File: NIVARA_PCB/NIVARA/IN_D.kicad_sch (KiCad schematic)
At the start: 0 parts

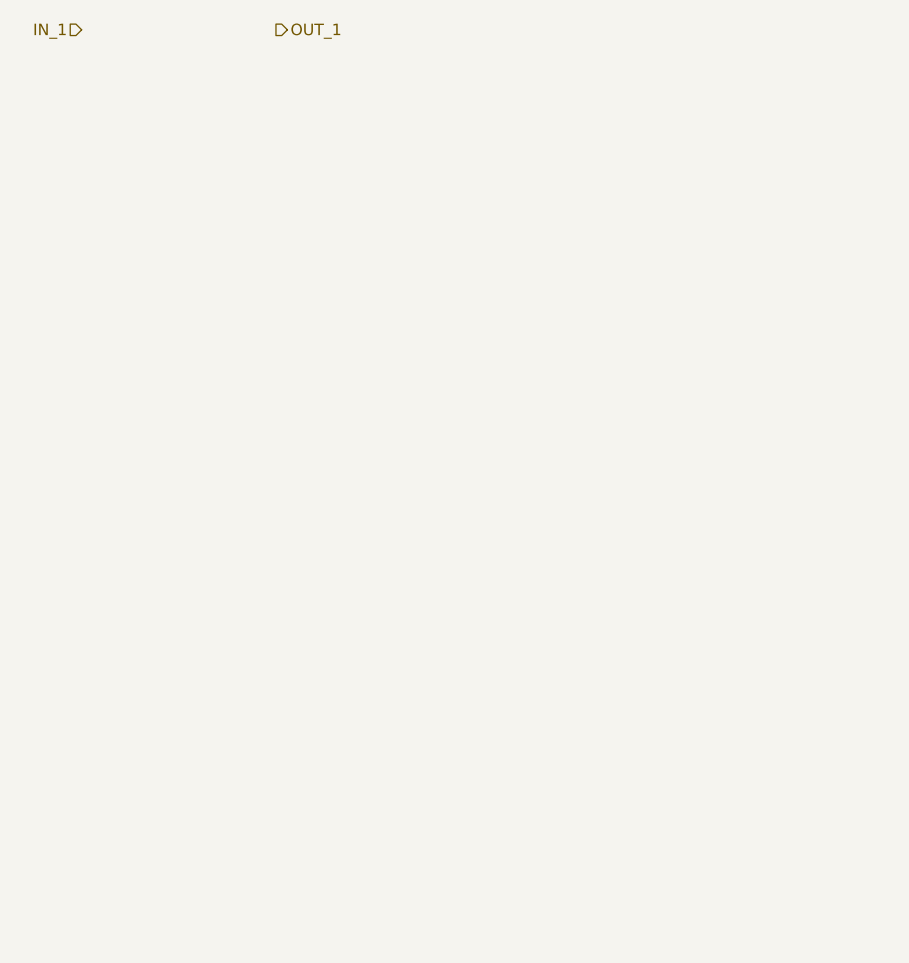
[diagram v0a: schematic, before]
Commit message: avance
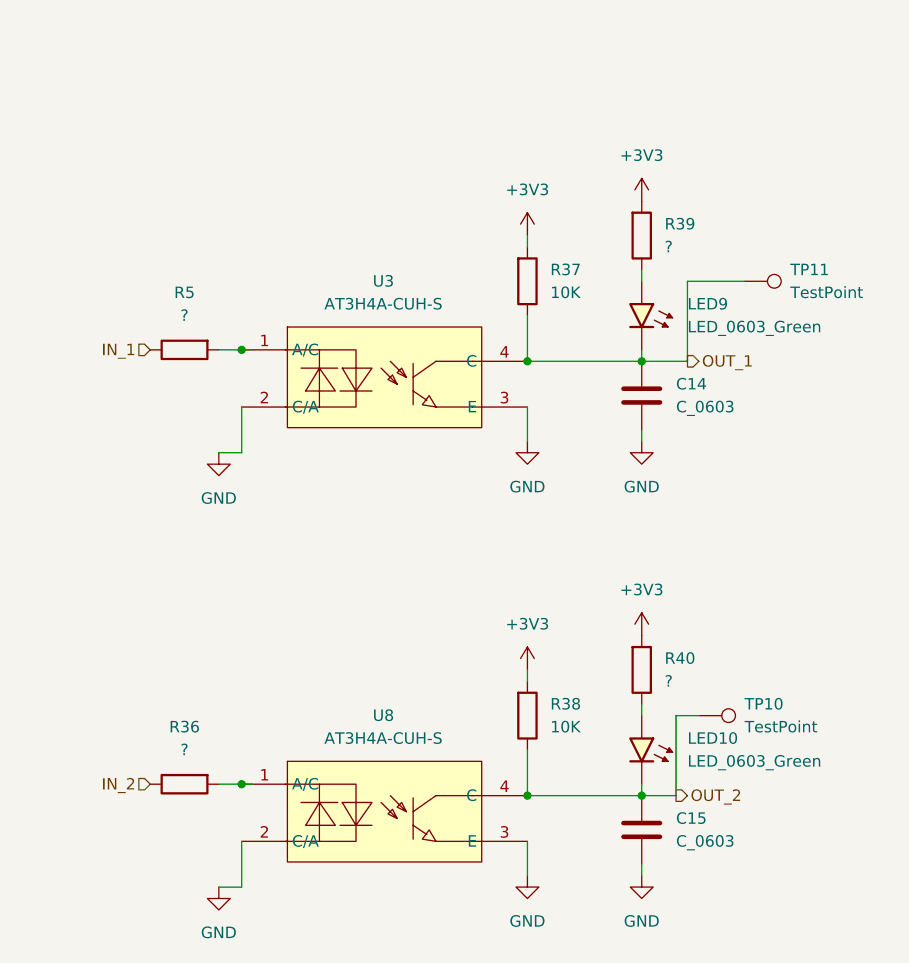
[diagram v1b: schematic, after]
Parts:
- added C14, C15: C_0603, PCM_Capacitor_SMD_AKL:C_0603_1608Metric, symbol PCM_Capacitor_AKL:C_0603
- added LED10, LED9: LED_0603_Green, PCM_LED_SMD_AKL:LED_0603_1608Metric, symbol PCM_LED_AKL:LED_0603_Green
- added R36, R5: ?, PCM_Resistor_SMD_AKL:R_1206_3216Metric_Pad1.30x1.75mm_HandSolder, symbol PCM_Resistor_AKL:R_0603
- added R37, R38: 10K, PCM_Resistor_SMD_AKL:R_0603_1608Metric, symbol PCM_Resistor_AKL:R_0603
- added R39, R40: ?, PCM_Resistor_SMD_AKL:R_0603_1608Metric, symbol PCM_Resistor_AKL:R_0603
- added TP10, TP11: TestPoint, TestPoint:TestPoint_THTPad_D1.0mm_Drill0.5mm, symbol Connector:TestPoint
- added U3, U8: AT3H4A-CUH-S, easyeda2kicad:SSOP-4_L2.7-W4.6-P1.27-LS7.0-TL, symbol easyeda2kicad:AT3H4A-CUH-S
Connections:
- net IN_1: now also R5.2
- net OUT_1: now also C14.1, LED9.1 (K), R37.2, TP11.1, U3.4 (C)
- new net: R5.1, U3.1 (A/C)
- new net: R36.1, U8.1 (A/C)
- new net: LED10.2 (A), R40.2
- new net: LED9.2 (A), R39.2
- new net +3V3: R37.1, R38.1, R39.1, R40.1
- new net GND: C14.2, C15.2, U3.2 (C/A), U3.3 (E), U8.2 (C/A), U8.3 (E)
- new net IN_2: R36.2
- new net OUT_2: C15.1, LED10.1 (K), R38.2, TP10.1, U8.4 (C)
